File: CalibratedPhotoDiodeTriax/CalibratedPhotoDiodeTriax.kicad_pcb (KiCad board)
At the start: 2 copper layers, 50.8 x 50.8 mm, 2 parts, among them J1 TO-5 Photodiode Socket: Conn_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, J2 CBJ70 Triax Throughhole Conne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

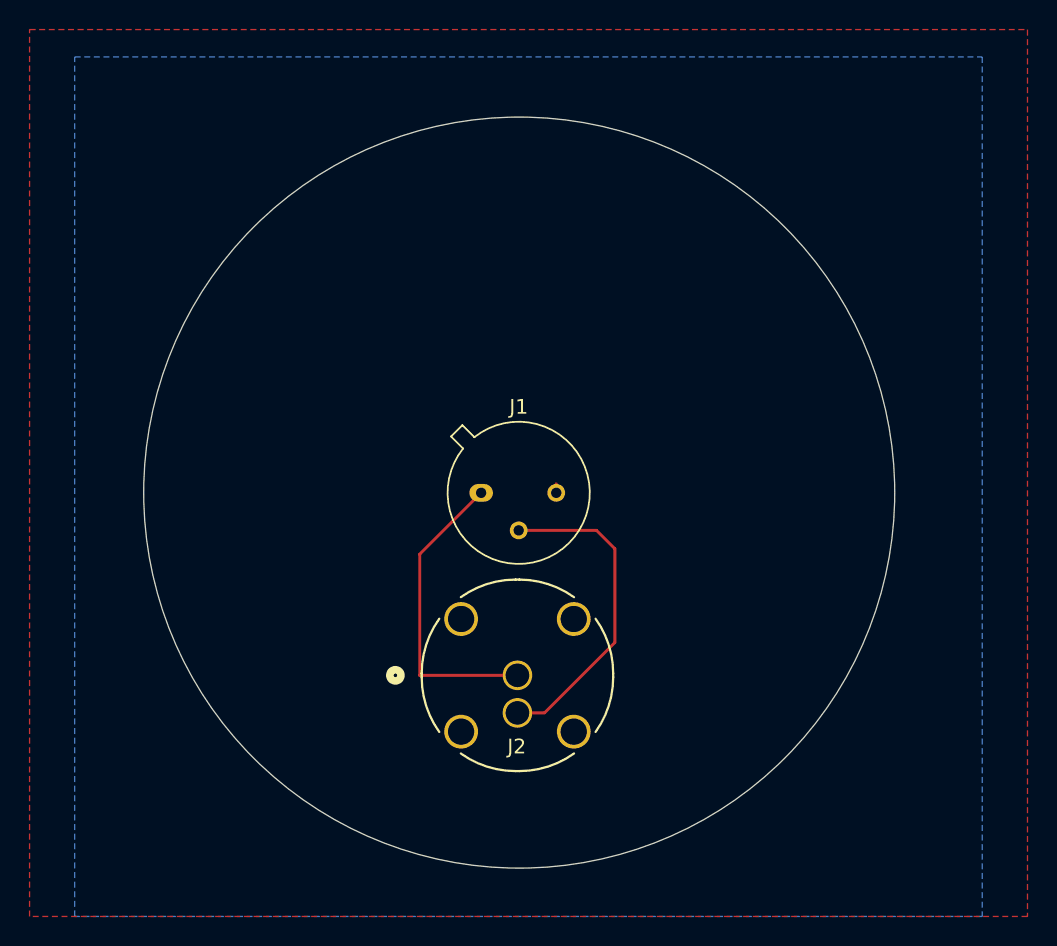
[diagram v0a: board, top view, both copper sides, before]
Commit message: Trying to revise accessibility
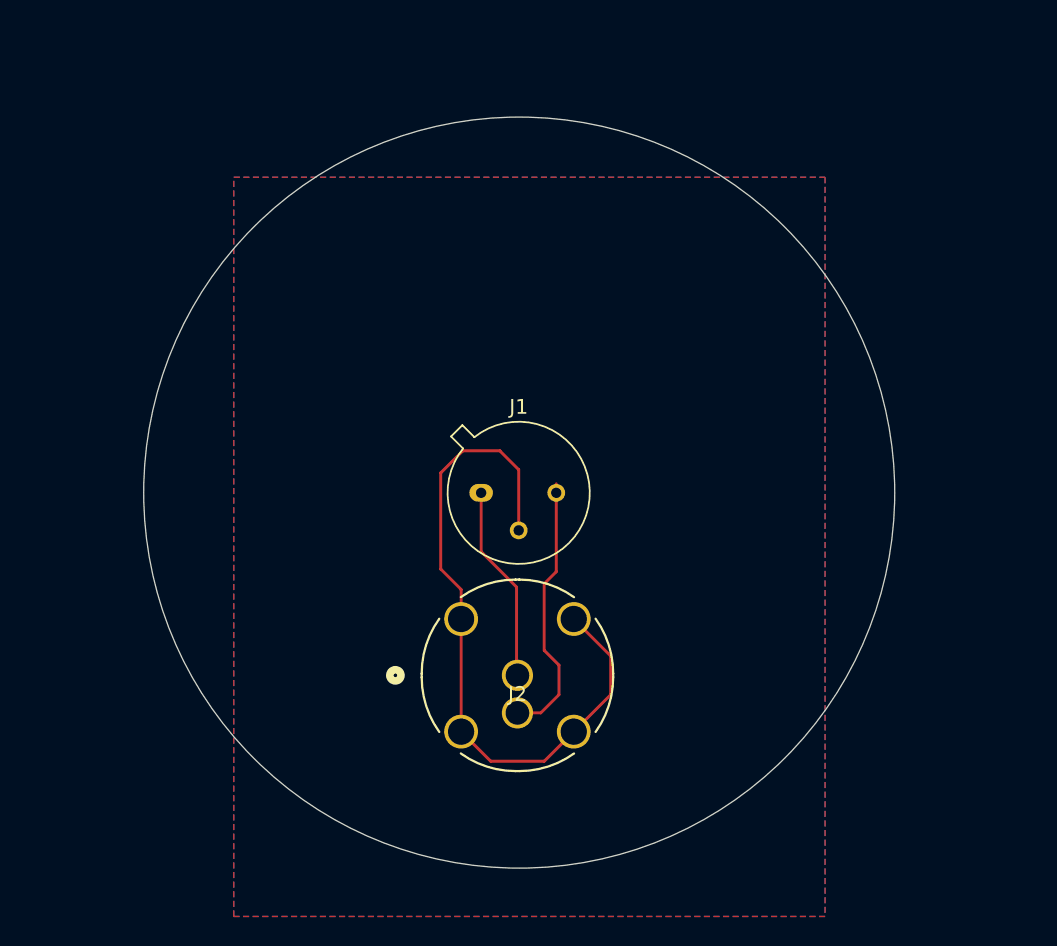
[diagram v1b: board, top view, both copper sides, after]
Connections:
- J1 pad 2: Net-(J1-Pin_2) -> GND
- J1 pad 3: GND -> Net-(J1-Pin_3)
- J2 pad 2: Net-(J1-Pin_2) -> Net-(J1-Pin_3)
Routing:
- net GND: track 0.61 -> 47.6 mm
- net Net-(J1-Pin_2): track 21.9 -> 0.00 mm
- net Net-(J1-Pin_3): track 0.00 -> 18.3 mm
- net Net-(J1-Pin_1): track 20.7 -> 13.2 mm
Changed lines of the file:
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@@
 	(net 0 "")
 	(net 1 "Net-(J1-Pin_1)")
-	(net 2 "Net-(J1-Pin_2)")
+	(net 2 "Net-(J1-Pin_3)")
 	(net 3 "GND")
 	(footprint "KiCADv6:CONN_CBJ70_CIN"
@@
 		(tags "CBJ70 ")
 		(property "Reference" "J2"
-			(at -0.05 4.82 0)
+			(at 0 1.27 0)
 			(unlocked yes)
 			(layer "F.SilkS")
@@
 		)
 		(property "Value" "CBJ70 Triax Throughhole Connector"
-			(at 0 7.7 0)
+			(at 0 8.19 0)
 			(unlocked yes)
 			(layer "F.Fab")
@@
 		)
 		(fp_text user "${REFERENCE}"
-			(at -0.07 4.8 0)
+			(at 0 1.27 0)
 			(unlocked yes)
 			(layer "F.Fab")
@@
 		(pad "1" thru_hole circle
 			(at 0 0)
-			(size 2 2)
-			(drill 1.6)
+			(size 2.1082 2.1082)
+			(drill 1.6002)
 			(layers "*.Cu" "*.Mask")
 			(remove_unused_layers no)
@@
 		(pad "2" thru_hole circle
 			(at 0 2.54)
-			(size 2 2)
-			(drill 1.6)
+			(size 2.1082 2.1082)
+			(drill 1.6002)
 			(layers "*.Cu" "*.Mask")
 			(remove_unused_layers no)
-			(net 2 "Net-(J1-Pin_2)")
+			(net 2 "Net-(J1-Pin_3)")
 			(pinfunction "In2")
 			(pintype "passive")
@@
 			(size 2.286 2.286)
 			(drill 1.778)
-			(layers "*.Cu" "*.Mask")
+			(layers "*.Cu" "*.Mask" "Dwgs.User")
 			(remove_unused_layers no)
 			(net 3 "GND")
@@
 			(layers "*.Cu" "*.Mask")
 			(remove_unused_layers no)
-			(net 2 "Net-(J1-Pin_2)")
+			(net 3 "GND")
 			(pinfunction "Pin_2")
 			(pintype "passive")
@@
 			(layers "*.Cu" "*.Mask")
 			(remove_unused_layers no)
-			(net 3 "GND")
+			(net 2 "Net-(J1-Pin_3)")
 			(pinfunction "Pin_3")
 			(pintype "passive")
@@
 			)
 		)
-	)
-	(gr_circle
-		(center 159.779612 71.39)
-		(end 160.479612 70.341869)
-		(stroke
-			(width 0.1)
-			(type solid)
-		)
-		(fill no)
-		(layer "F.Mask")
-	)
-	(gr_circle
-		(center 159.69 81.179612)
-		(end 160.39 80.131481)
-		(stroke
-			(width 0.1)
-			(type solid)
-		)
-		(fill no)
-		(layer "F.Mask")
-	)
-	(gr_circle
-		(center 157.239612 68.848895)
-		(end 157.939612 67.800764)
-		(stroke
-			(width 0.1)
-			(type solid)
-		)
-		(fill no)
-		(layer "F.Mask")
-	)
-	(gr_circle
-		(center 159.69 83.719612)
-		(end 160.39 82.671481)
-		(stroke
-			(width 0.1)
-			(type solid)
-		)
-		(fill no)
-		(layer "F.Mask")
-	)
-	(gr_circle
-		(center 159.779612 71.38)
-		(end 160.479612 70.331869)
-		(stroke
-			(width 0.1)
-			(type solid)
-		)
-		(fill no)
-		(layer "B.Mask")
-	)
-	(gr_circle
-		(center 157.239612 68.848895)
-		(end 157.939612 67.800764)
-		(stroke
-			(width 0.1)
-			(type solid)
-		)
-		(fill no)
-		(layer "B.Mask")
-	)
-	(gr_circle
-		(center 159.69 83.719612)
-		(end 160.39 82.671481)
-		(stroke
-			(width 0.1)
-			(type default)
-		)
-		(fill no)
-		(layer "B.Mask")
-	)
-	(gr_circle
-		(center 159.69 81.179612)
-		(end 160.39 80.131481)
-		(stroke
-			(width 0.1)
-			(type default)
-		)
-		(fill no)
-		(layer "B.Mask")
 	)
 	(gr_circle
@@
 	)
 	(segment
-		(start 153.08 72.9998)
-		(end 153.08 81.19)
+		(start 157.235 72.825)
+		(end 159.63 75.22)
 		(width 0.2)
 		(layer "F.Cu")
@@
 	(segment
 		(start 157.235 68.8448)
-		(end 153.08 72.9998)
+		(end 157.235 72.825)
 		(width 0.2)
 		(layer "F.Cu")
@@
 	)
 	(segment
-		(start 153.08 81.19)
-		(end 159.69 81.19)
+		(start 159.63 75.22)
+		(end 159.63 81.03)
 		(width 0.2)
 		(layer "F.Cu")
@@
 	)
 	(segment
-		(start 159.775 71.3848)
-		(end 165.0348 71.3848)
+		(start 162.5 80.5)
+		(end 162.5 82.5)
 		(width 0.2)
 		(layer "F.Cu")
@@
 	)
 	(segment
-		(start 161.52 83.73)
-		(end 159.69 83.73)
+		(start 162.315 74.185)
+		(end 161.5 75)
 		(width 0.2)
 		(layer "F.Cu")
@@
 	)
 	(segment
-		(start 166.28 72.63)
-		(end 166.28 78.97)
+		(start 161.5 75)
+		(end 161.5 79.5)
 		(width 0.2)
 		(layer "F.Cu")
@@
 	)
 	(segment
-		(start 166.28 78.97)
-		(end 161.52 83.73)
-		(width 0.2)
-		(layer "F.Cu")
-		(net 2)
-	)
-	(segment
-		(start 165.0348 71.3848)
-		(end 166.28 72.63)
+		(start 161.5 79.5)
+		(end 162.5 80.5)
 		(width 0.2)
 		(layer "F.Cu")
@@
 		(width 0.2)
 		(layer "F.Cu")
+		(net 2)
+	)
+	(segment
+		(start 162.5 82.5)
+		(end 161.27 83.73)
+		(width 0.2)
+		(layer "F.Cu")
+		(net 2)
+	)
+	(segment
+		(start 161.27 83.73)
+		(end 159.69 83.73)
+		(width 0.2)
+		(layer "F.Cu")
+		(net 2)
+	)
+	(segment
+		(start 162.315 68.8448)
+		(end 162.315 74.185)
+		(width 0.2)
+		(layer "F.Cu")
+		(net 2)
+	)
+	(segment
+		(start 159.775 71.3848)
+		(end 159.775 67.275)
+		(width 0.2)
+		(layer "F.Cu")
+		(net 3)
+	)
+	(segment
+		(start 158.5 66)
+		(end 156 66)
+		(width 0.2)
+		(layer "F.Cu")
+		(net 3)
+	)
+	(segment
+		(start 154.5 67.5)
+		(end 154.5 74)
+		(width 0.2)
+		(layer "F.Cu")
+		(net 3)
+	)
+	(segment
+		(start 161.5 87)
+		(end 163.5 85)
+		(width 0.2)
+		(layer "F.Cu")
+		(net 3)
+	)
+	(segment
+		(start 163.5 85)
+		(end 166 82.5)
+		(width 0.2)
+		(layer "F.Cu")
+		(net 3)
+	)
+	(segment
+		(start 155.88 75.38)
+		(end 155.88 77.38)
+		(width 0.2)
+		(layer "F.Cu")
+		(net 3)
+	)
+	(segment
+		(start 155.88 77.38)
+		(end 155.88 85)
+		(width 0.2)
+		(layer "F.Cu")
+		(net 3)
+	)
+	(segment
+		(start 159.775 67.275)
+		(end 158.5 66)
+		(width 0.2)
+		(layer "F.Cu")
+		(net 3)
+	)
+	(segment
+		(start 154.5 74)
+		(end 155.88 75.38)
+		(width 0.2)
+		(layer "F.Cu")
+		(net 3)
+	)
+	(segment
+		(start 156 66)
+		(end 154.5 67.5)
+		(width 0.2)
+		(layer "F.Cu")
+		(net 3)
+	)
+	(segment
+		(start 166 79.88)
+		(end 163.5 77.38)
+		(width 0.2)
+		(layer "F.Cu")
+		(net 3)
+	)
+	(segment
+		(start 155.88 85)
+		(end 157.88 87)
+		(width 0.2)
+		(layer "F.Cu")
+		(net 3)
+	)
+	(segment
+		(start 166 82.5)
+		(end 166 79.88)
+		(width 0.2)
+		(layer "F.Cu")
+		(net 3)
+	)
+	(segment
+		(start 157.88 87)
+		(end 161.5 87)
+		(width 0.2)
+		(layer "F.Cu")
 		(net 3)
 	)
@@
 		(hatch edge 0.5)
 		(connect_pads
-			(clearance 0.05)
-		)
-		(min_thickness 0.1)
+			(clearance 0.5)
+		)
+		(min_thickness 0.25)
 		(filled_areas_thickness no)
 		(fill yes
@@
 		(polygon
 			(pts
-				(xy 126.69 37.51) (xy 194.19 37.51) (xy 194.19 97.5) (xy 126.69 97.5)
+				(xy 140.5 47.5) (xy 180.5 47.5) (xy 180.5 97.5) (xy 140.5 97.5)
 			)
 		)
@@
 		(priority 1)
 		(connect_pads
-			(clearance 0.05)
-		)
-		(min_thickness 0.1)
+			(clearance 0.5)
+		)
+		(min_thickness 0.25)
 		(filled_areas_thickness no)
 		(fill yes
@@
 		(polygon
 			(pts
-				(xy 129.74 39.36) (xy 191.13 39.36) (xy 191.13 97.5) (xy 129.74 97.5)
-			)
-		)
+				(xy 140.5 47.5) (xy 180.5 47.5) (xy 180.5 97.5) (xy 140.5 97.5)
+			)
+		)
